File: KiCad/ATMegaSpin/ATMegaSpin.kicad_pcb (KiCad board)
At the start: 2 copper layers, 100.2 x 139 mm, 30 parts, among them X1 ED281DT, Y1 ECS-160-18-4X-CKM

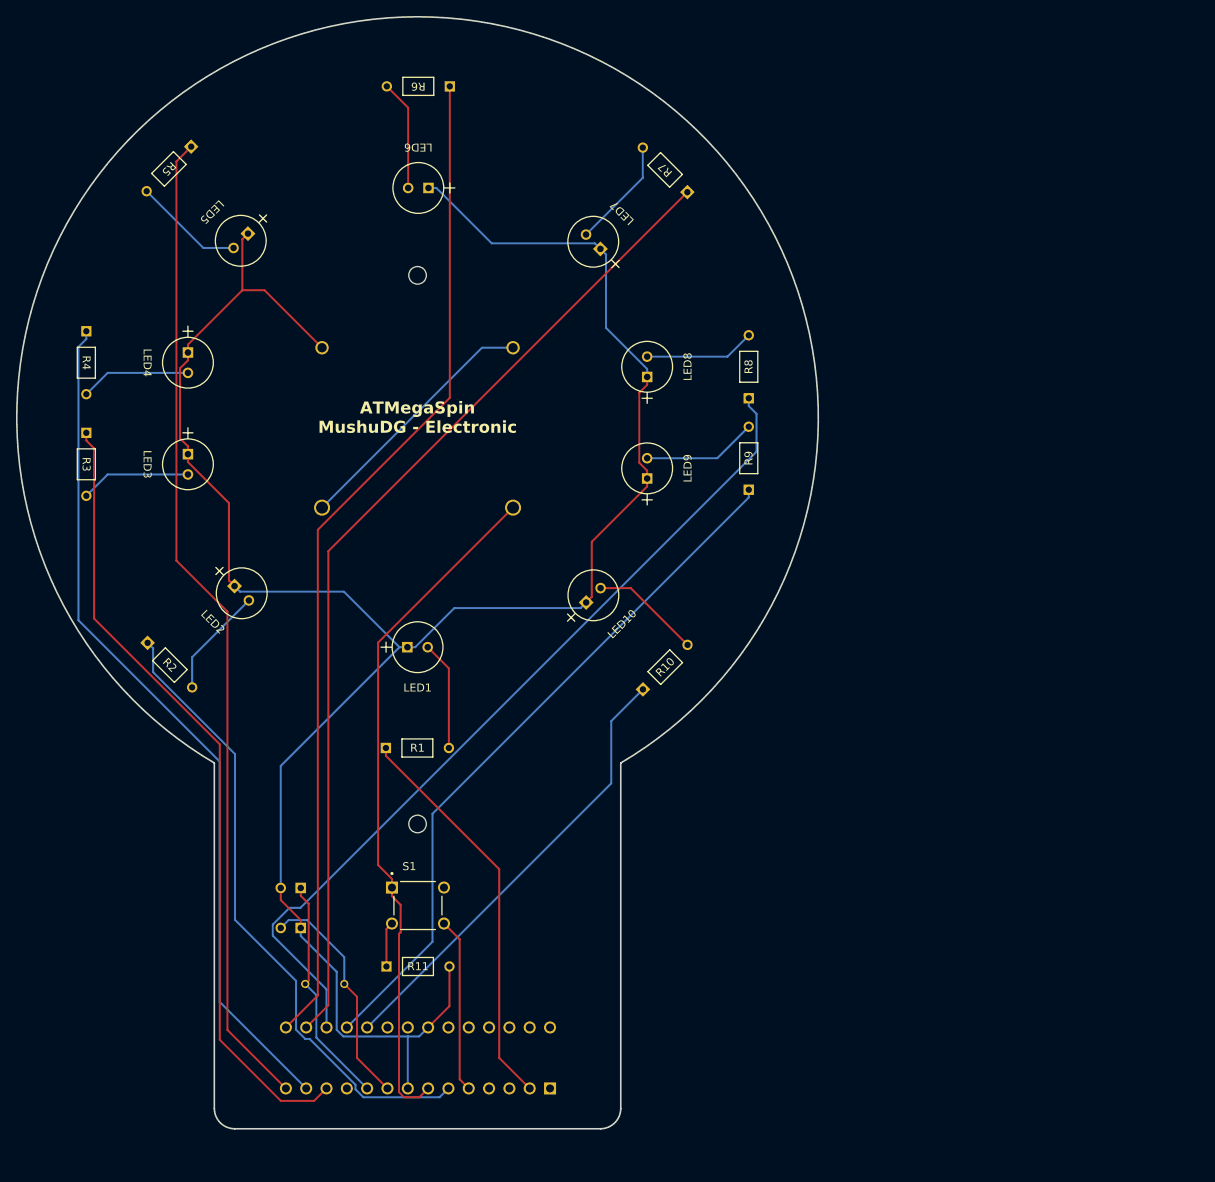
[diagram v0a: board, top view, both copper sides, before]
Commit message: Adapt tree
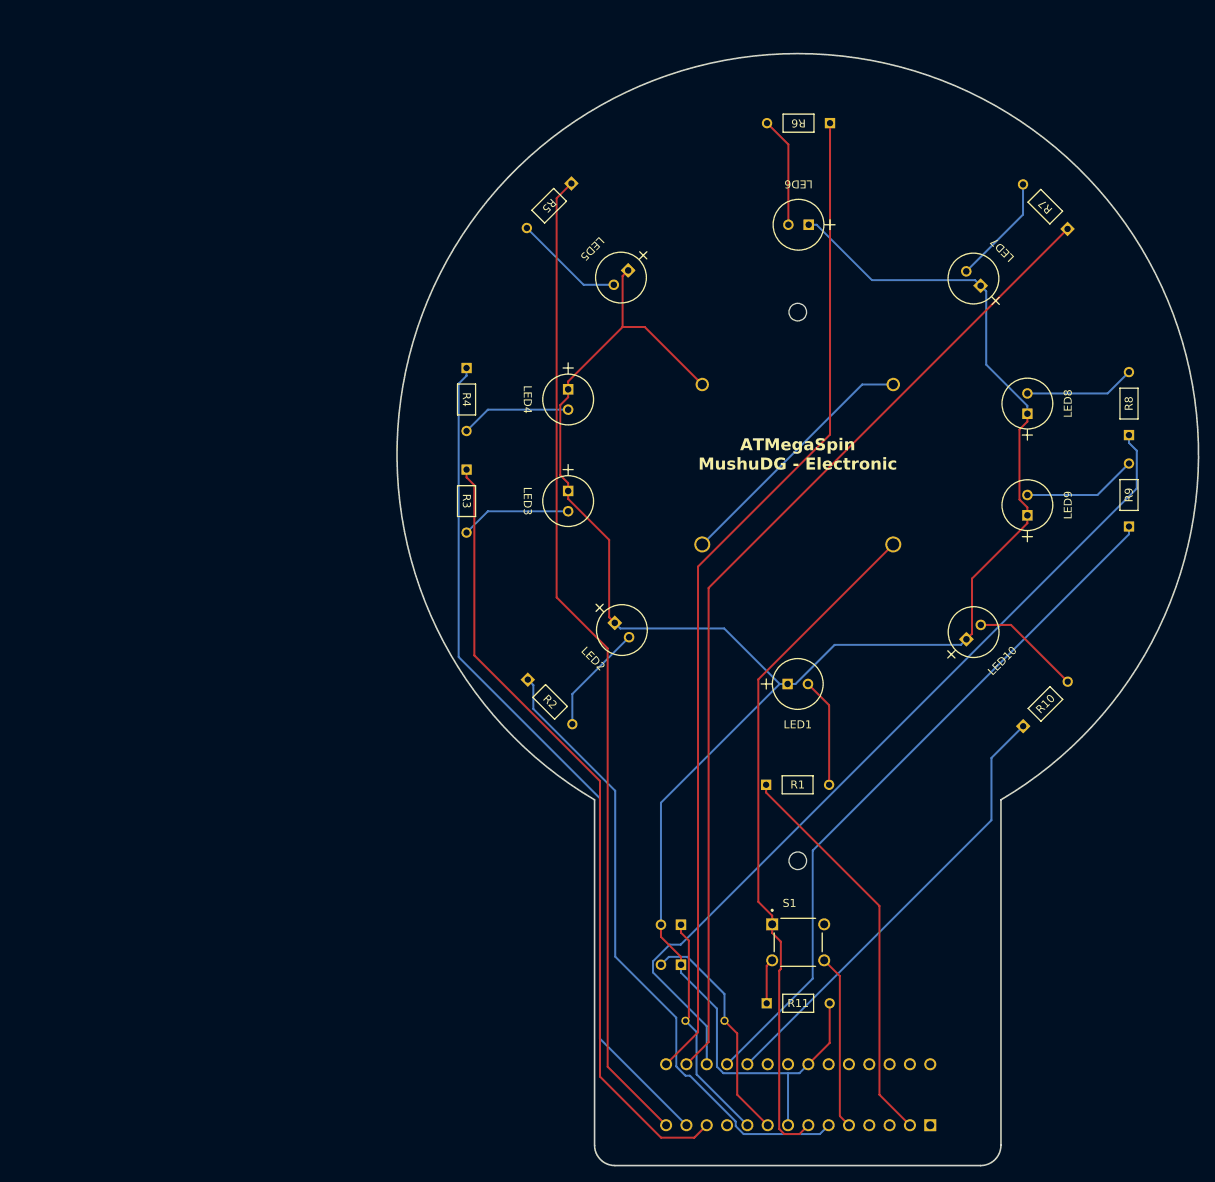
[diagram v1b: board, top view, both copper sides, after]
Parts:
- moved LED8 47.7 mm to (177.8, 75.7)
- moved LED9 47.7 mm to (177.8, 88.4)
- moved R10 47.7 mm to (177.3, 114.8)
- moved R7 47.7 mm to (182.9, 52.6)
- moved REF** 47.7 mm to (149.1, 131.6)
- moved REF** 47.7 mm to (149.1, 63.0)
- moved B1 47.7 mm to (161.1, 72.1)
- moved LED1 47.7 mm to (147.9, 109.5)
- moved LED10 47.7 mm to (170.2, 103.9)
- moved LED2 47.7 mm to (126.2, 101.9)
- moved LED3 47.7 mm to (120.4, 85.4)
- moved LED4 47.7 mm to (120.4, 72.7)
- moved LED5 47.7 mm to (127.9, 57.8)
- moved LED6 47.7 mm to (150.5, 52.1)
- moved LED7 47.7 mm to (172.0, 59.7)
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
